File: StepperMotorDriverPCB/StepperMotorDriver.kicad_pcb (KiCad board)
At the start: 4 copper layers, 44 x 39.2 mm, 66 parts, among them IC2 TMC2209-LA, J1 Conn_01x02_Pin, J10 USB_C_Receptacle_USB2.0_16P, J2 Conn_01x01_Pin, J3 Conn_01x01_Pin, J4 Conn_01x04_Socket, J7 Conn_01x02_Pin, J8 Conn_01x01_Pin, J9 Conn_01x01_Pin, SW1 SW_SPST, SW2 SW_SPST, U2 SN65HVD232, U3 STM32G473CBTx, U5 AP63203WU, U6 MT6701CT, Y2 16MHz

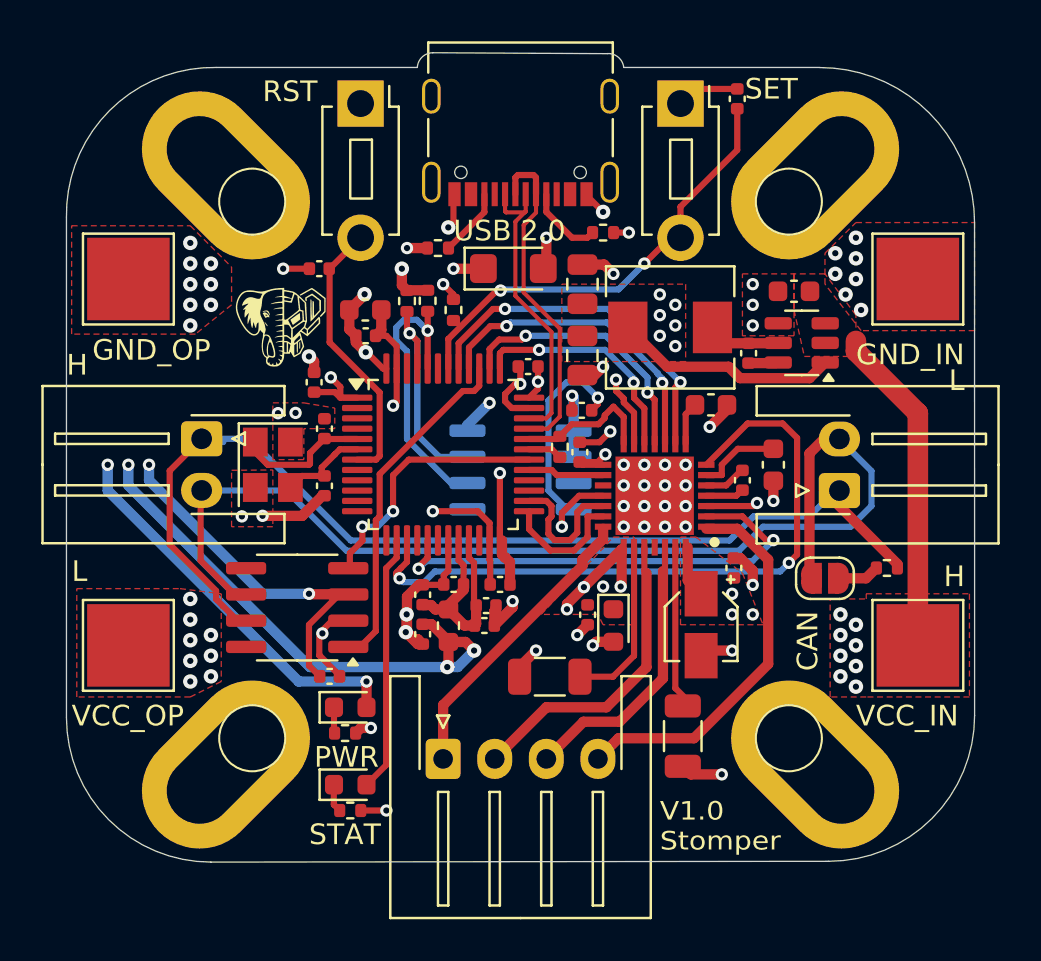
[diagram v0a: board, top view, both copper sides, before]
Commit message: Updates to circuitry
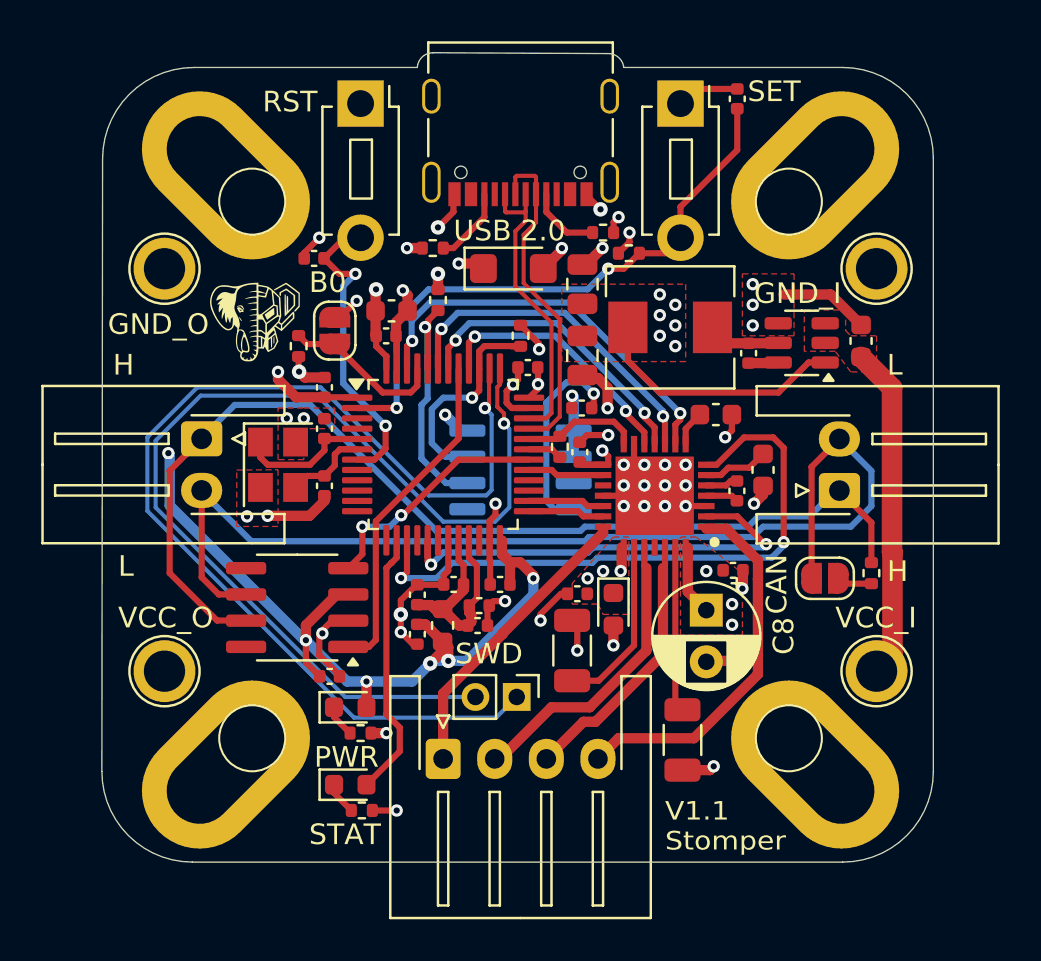
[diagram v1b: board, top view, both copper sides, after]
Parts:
- added J5: Conn_01x02_Pin, Connector_PinHeader_2.00mm:PinHeader_1x02_P2.00mm_Vertical, F.Cu at (73.1, 73.8)
- added JP2: Jumper_2_Bridged, Jumper:SolderJumper-2_P1.3mm_Open_RoundedPad1.0x1.5mm, F.Cu at (64.2, 56.0)
- added R12: 10k, Resistor_SMD:R_0402_1005Metric, F.Cu at (62.5, 56.8)
- C8: footprint Capacitor_SMD:CP_Elec_3x5.3 -> Capacitor_THT:CP_Radial_D5.0mm_P2.50mm
- J2, J3, J8, J9: footprint TestPoint:TestPoint_Pad_4.0x4.0mm -> TestPoint:TestPoint_Plated_Hole_D2.0mm
- R1: value 1k5 -> 10k
- moved R1 8.93 mm to (78.5, 52.2), turned to 0 degrees
- moved R2 5.75 mm to (73.2, 56.2)
- moved C25 4.04 mm to (89.8, 56.5), turned to -90 degrees
- moved J3 2.36 mm to (90.5, 72.5)
- moved J8 2.15 mm to (56.0, 72.5)
- moved J9 2.06 mm to (90.5, 53.0)
- moved J2 1.82 mm to (56.0, 53.0)
- moved R6 1.67 mm to (75.8, 71.5), turned to -90 degrees
- moved G*** 1.27 mm to (60.5, 55.5)
- moved C15 1.27 mm to (67.0, 55.0)
- moved C9 1.13 mm to (76.0, 68.8), turned to 180 degrees
- moved C16 0.99 mm to (66.7, 56.3)
- moved R11 0.79 mm to (90.2, 67.8), turned to 90 degrees
- moved D2 0.79 mm to (77.8, 69.5)
- moved R9 0.75 mm to (65.5, 75.5)
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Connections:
- U3 pad 2: unconnected-(U3-PC13-Pad2) -> Net-(SW1-B)
- U3 pad 37: /MOT_INDEX -> /SWDIO
- U3 pad 38: /MOT_DIAG -> /SWCLK
- U3 pad 39: /CAN_TX -> /ESCL
- U3 pad 40: /MOT_MS2 -> /MOT_INDEX
- U3 pad 41: /MOT_MS1 -> /CAN_TX
- U3 pad 42: Net-(SW1-B) -> /MOT_DIAG
- U3 pad 43: unconnected-(U3-PB6-Pad43) -> /MOT_MS2
- U3 pad 45: /ESCL -> Net-(JP2-B)
- U3 pad 46: unconnected-(U3-PB9-Pad46) -> /MOT_MS1
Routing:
- net /SWCLK: track 0.00 -> 52.1 mm, vias 0 -> 1
- net /SWDIO: track 0.00 -> 50.4 mm, vias 0 -> 1
- net +3V3: track 102.1 -> 78.2 mm, vias 24 -> 23
- net Net-(JP2-B): track 0.00 -> 7.88 mm
- net Net-(SW1-B): track 22.1 -> 29.4 mm
- net GND: track 82.5 -> 89.7 mm, vias 68 -> 46
- net VCC: track 25.3 -> 21.8 mm, vias 24 -> 7
- net /MOT_DIR: track 6.65 -> 3.69 mm
- net /MOT_SPREAD: track 33.2 -> 30.4 mm
- net /MOT_STBY: track 6.15 -> 3.69 mm
- net /MOT_MS1: track 17.3 -> 19.6 mm
- net Net-(SW2-B): track 13.9 -> 15.7 mm, vias 0 -> 2
- net /ESDA: track 14.1 -> 12.4 mm
- net /MOT_DIAG: track 13.1 -> 14.7 mm
- net /MOT_MS2: track 15.3 -> 16.7 mm
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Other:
- board size 44 x 39.2 mm -> 40.3 x 39.2 mm
- board text added: "B0"
- board text added: "CLK IO"
- board text added: "GND_I"
- board text added: "GND_O"
- board text added: "JoKhann 09/15/24"
- board text added: "SWD"
- board text added: "V1.1 Stomper"
- board text added: "VCC_I"
- board text added: "VCC_O"
- board text removed: "GND_IN"
- board text removed: "GND_OP"
- board text removed: "JoKhann 08/29/24"
- board text removed: "V1.0 Stomper"
- board text removed: "VCC_IN"
- board text removed: "VCC_OP"
